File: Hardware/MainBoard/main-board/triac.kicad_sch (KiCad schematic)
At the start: 18 parts, among them J4 Conn_01x03, J5 1366005, U2 DS18B20+, U3 MOC3083S-TA1

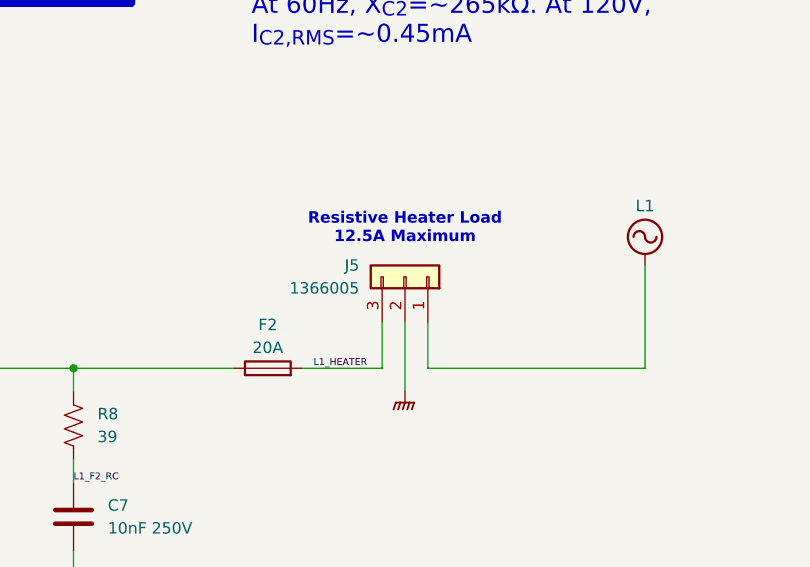
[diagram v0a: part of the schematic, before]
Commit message: Finish board layout
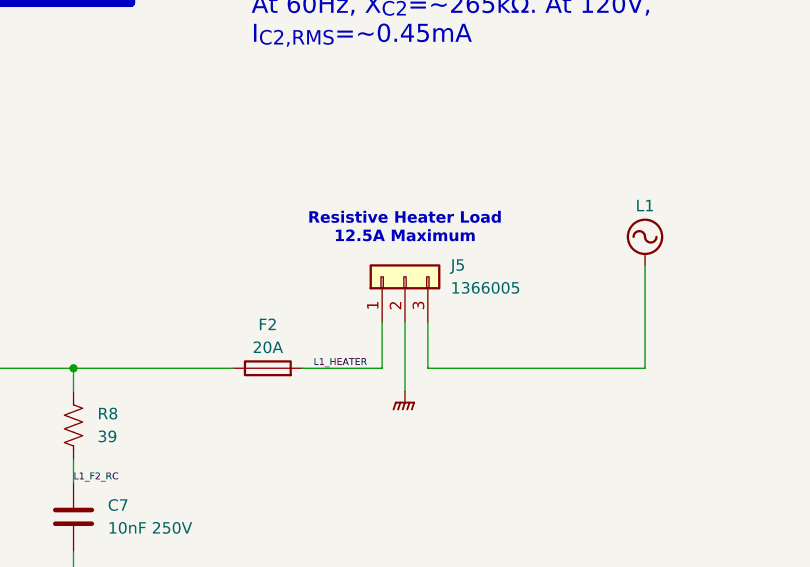
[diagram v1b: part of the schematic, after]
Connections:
- net L1: now also J5.3 (Pin_3); no longer J5.1 (Pin_1)
- net L1_HEATER: now also J5.1 (Pin_1); no longer J5.3 (Pin_3)
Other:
- moved on the sheet: J5
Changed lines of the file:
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@@
 	(symbol
 		(lib_id "Connector_Generic:Conn_01x03")
-		(at 303.53 104.14 270)
-		(mirror x)
+		(at 303.53 104.14 90)
 		(unit 1)
 		(exclude_from_sim no)
@@
 		(dnp no)
 		(property "Reference" "J5"
-			(at 298.45 102.8699 90)
+			(at 308.61 102.8699 90)
 			(effects
 				(font
@@
 		)
 		(property "Value" "1366005"
-			(at 298.45 105.4099 90)
+			(at 308.61 105.4099 90)
 			(effects
 				(font
